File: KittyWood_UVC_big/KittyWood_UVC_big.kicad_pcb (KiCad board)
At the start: 2 copper layers, 2 parts, among them K1 Wiper control relay, Q1 PN2222A

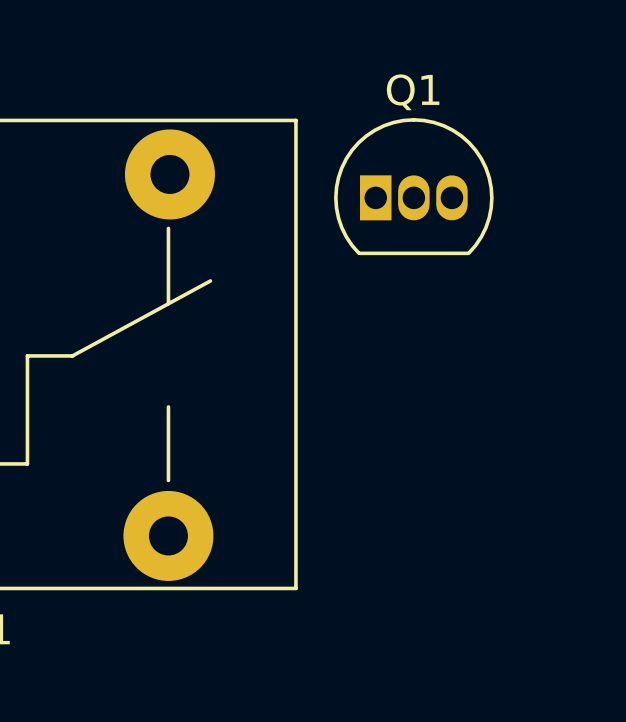
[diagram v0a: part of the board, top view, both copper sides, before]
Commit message: Updated PCB
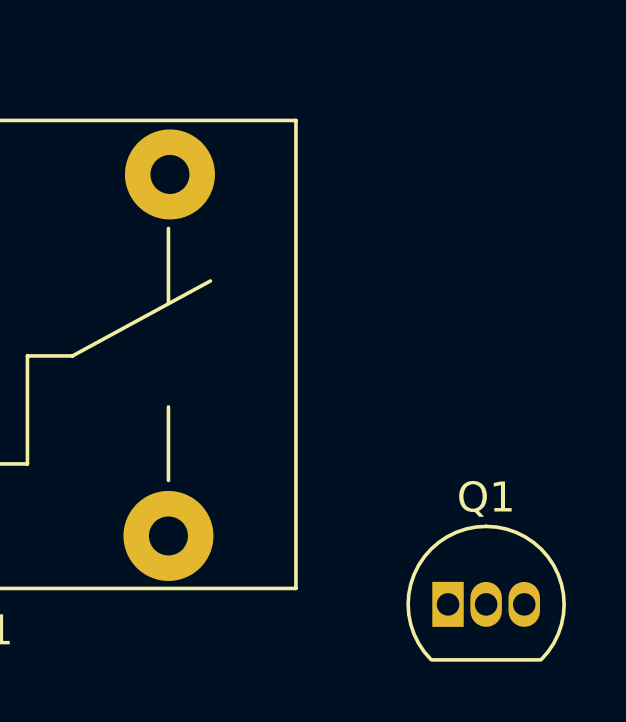
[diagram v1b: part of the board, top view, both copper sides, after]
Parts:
- moved Q1 13.8 mm to (116.9, 78.7)
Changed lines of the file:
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@@
   )
   (module "Package_TO_SOT_THT:TO-92_Inline" (layer "F.Cu")
-    (at 114.4812 65.138)
+    (at 116.8908 78.6892)
     (descr "TO-92 leads in-line, narrow, oval pads, drill 0.75mm (see NXP sot054_po.pdf)")
     (tags "to-92 sc-43 sc-43a sot54 PA33 transistor")

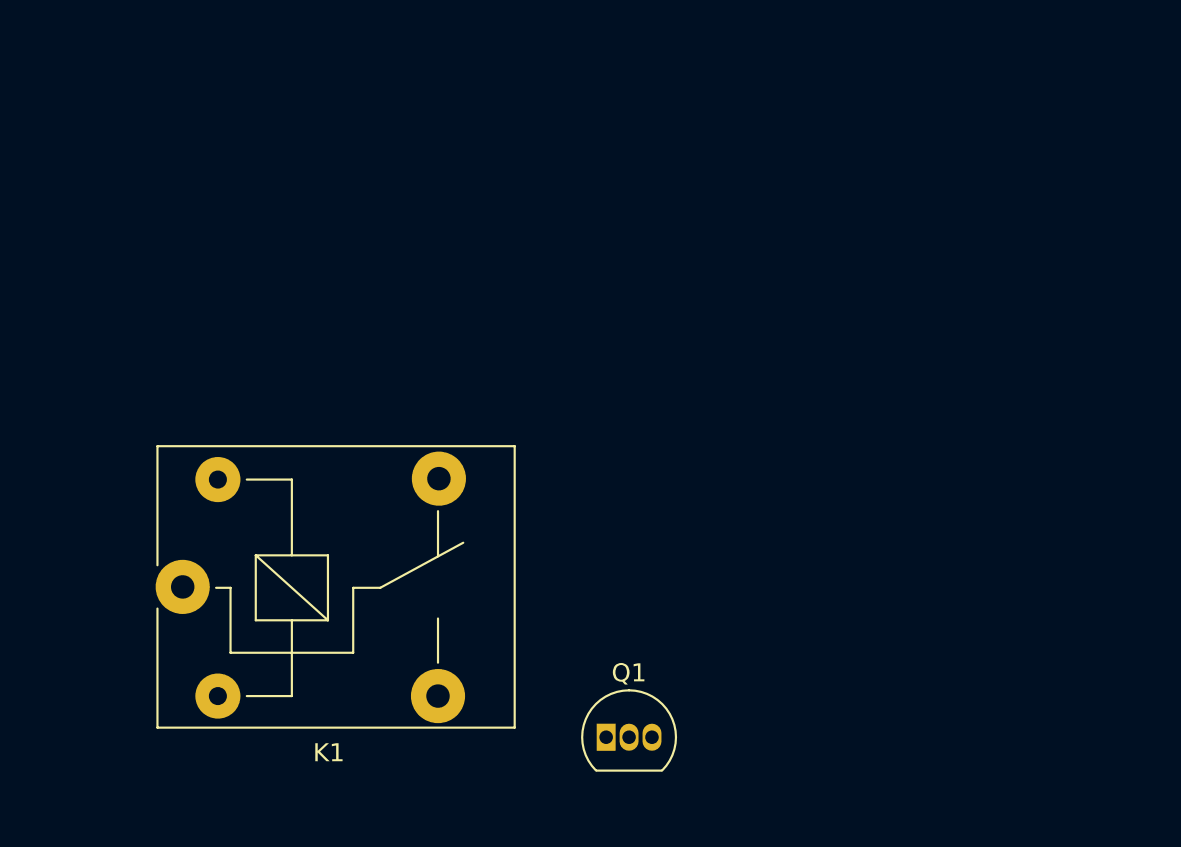
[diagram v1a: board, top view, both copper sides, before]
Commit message: test
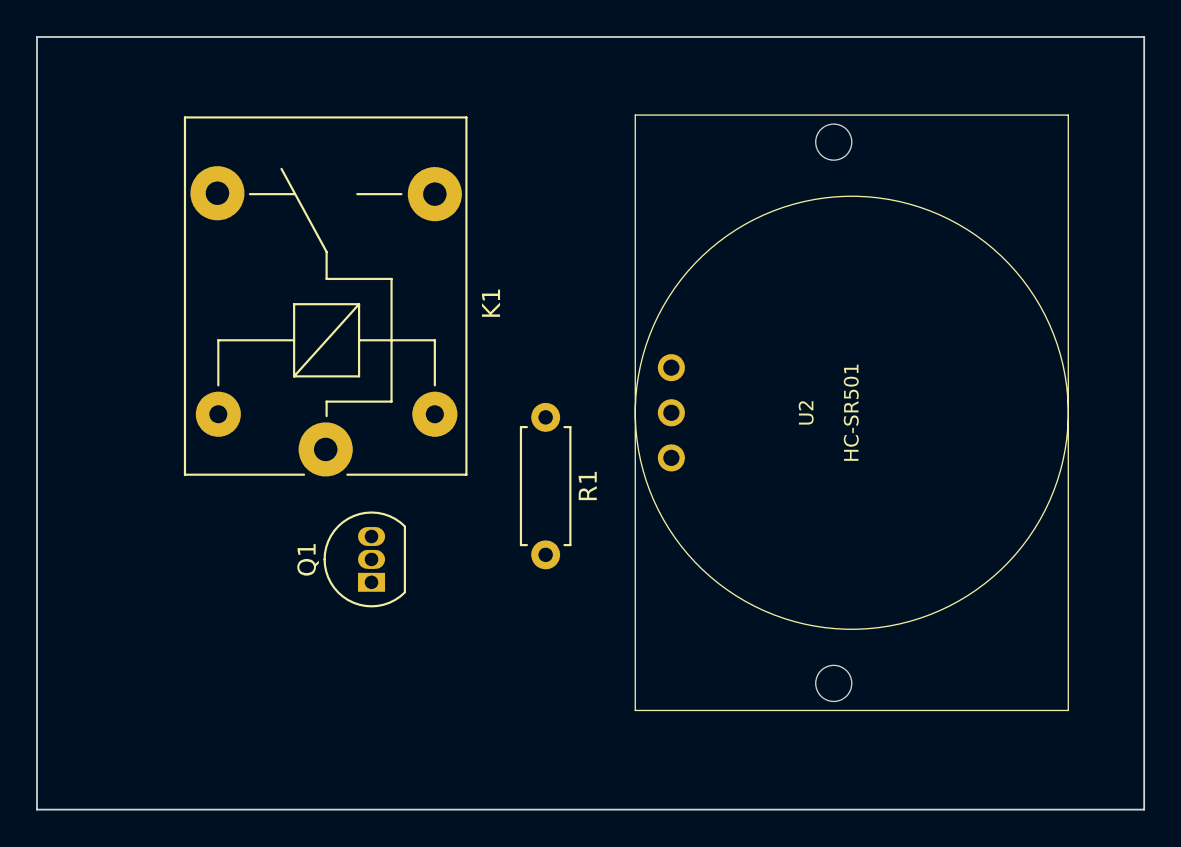
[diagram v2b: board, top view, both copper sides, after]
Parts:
- added R1: 10k, Resistor_THT:R_Axial_DIN0207_L6.3mm_D2.5mm_P7.62mm_Horizontal, F.Cu at (113.5, 61.0)
- added U2: HC-SR501, HC-SR501:HC-SR501, F.Cu at (130.5, 60.7)
- moved Q1 15.6 mm to (103.9, 70.1), turned to 90 degrees
- moved K1 11.0 mm to (101.3, 62.7), turned to 90 degrees
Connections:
- K1 pad 5: /12V -> +5V
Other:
- board outline added: 61.4 x 42.8 mm
